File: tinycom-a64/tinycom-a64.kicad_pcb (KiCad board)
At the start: 4 copper layers, 41.7 x 40.9 mm, 28 parts, among them P1 CONN_02X10, P2 CONN_02X10, U1 AllWinner-A64(FBGA396), U2 H5TQG63BFR/FBGA96, Y1 Crystal

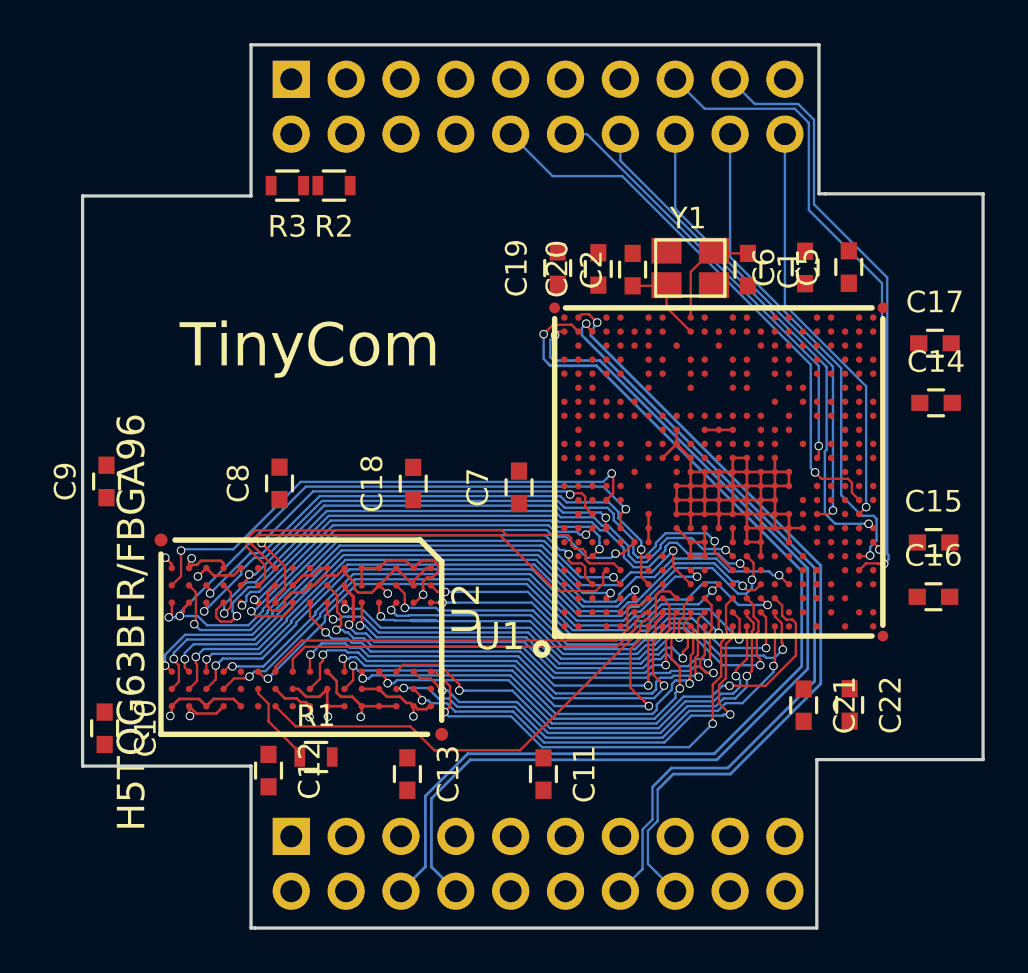
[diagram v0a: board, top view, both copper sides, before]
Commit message: route
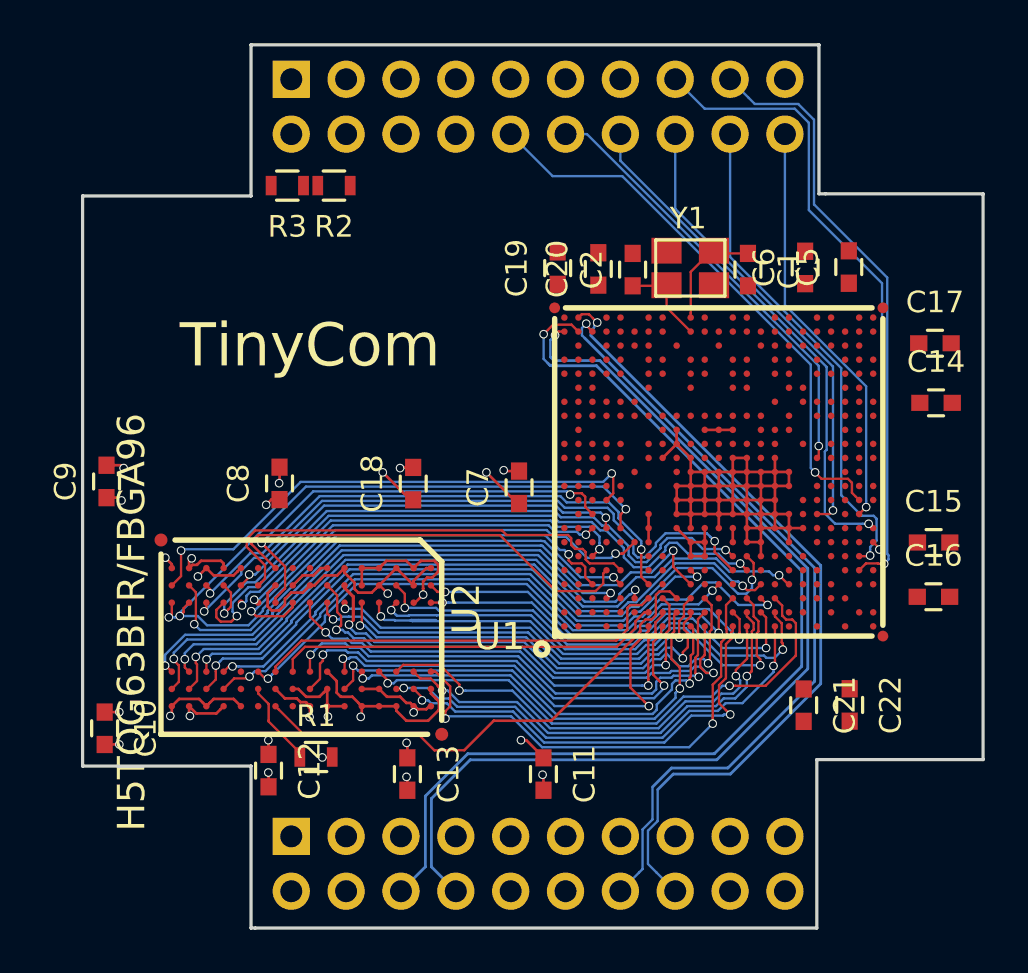
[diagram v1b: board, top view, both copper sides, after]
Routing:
- net VCC_15: track 30.4 -> 43.2 mm, vias 5 -> 13
- net GND: track 76.5 -> 82.4 mm, vias 6 -> 15
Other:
- net class Default: clearance 0.15 -> 0.125; trace_width 0.15 -> 0.125
- rule trace_clearance: 0.15 -> 0.125
